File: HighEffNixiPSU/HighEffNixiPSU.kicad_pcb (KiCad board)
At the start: 4 copper layers, 79.9 x 139.9 mm, 74 parts, among them IC1 AZ1117CH-3.3TRG1, J1 Jack-DC, J2 USB_C_Receptacle_USB2.0, Q1 FQD16N25CTM, Q10 2N2219, Q11 2N2219, Q2 2N2219, Q3 2N2219, Q4 2N2219, Q5 2N2219, Q6 2N2219, Q7 2N2219, Q8 2N2219, Q9 2N2219, SW2 EN, U1 LM3478MM, U2 ESP32-S3-MINI-1, U4 HV5622PG, U5 HV5622PG

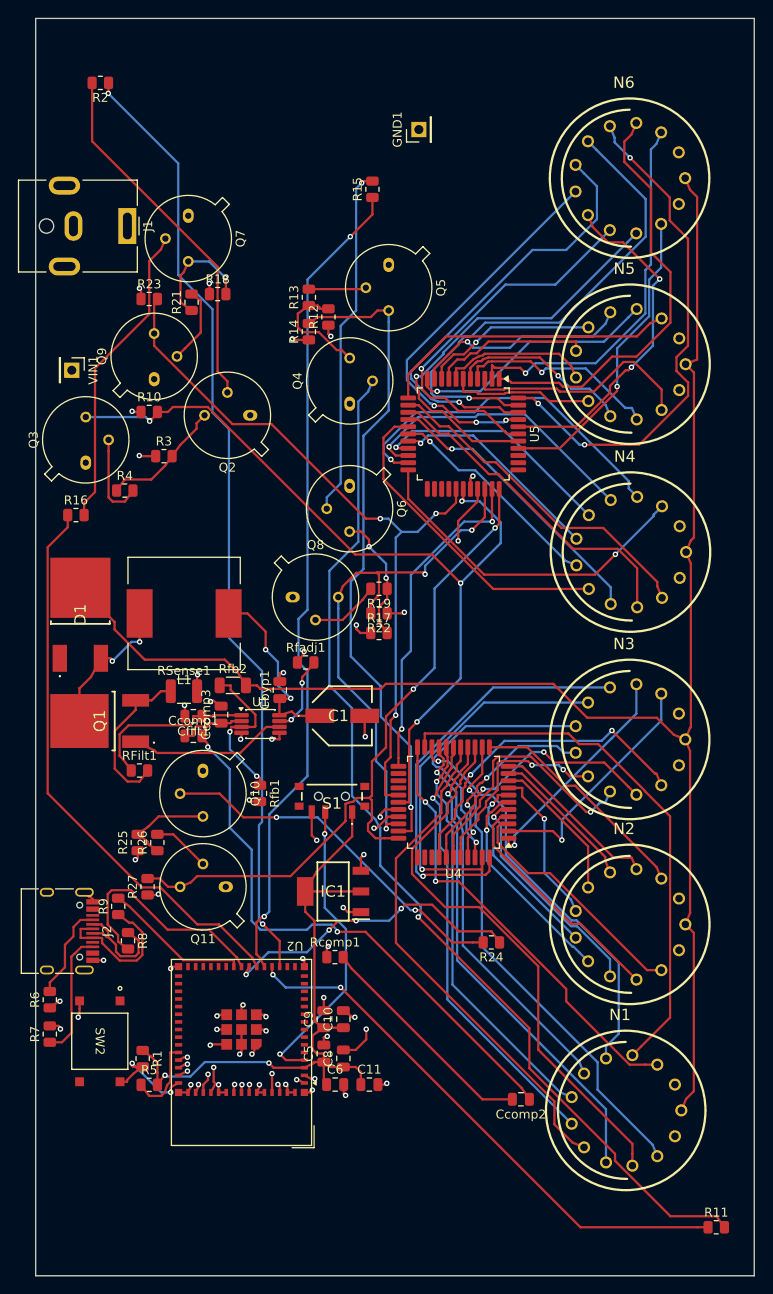
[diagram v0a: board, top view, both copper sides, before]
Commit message: afawj
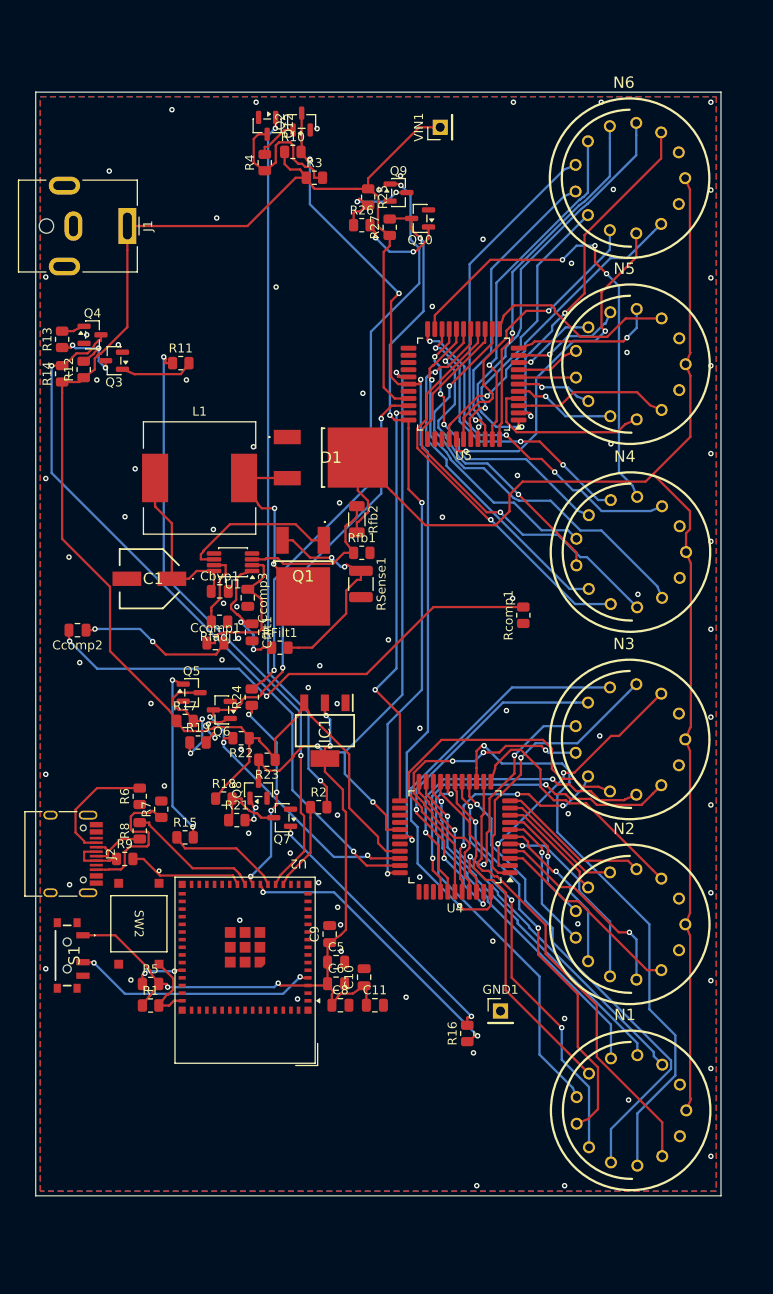
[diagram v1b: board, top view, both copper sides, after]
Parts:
- removed Q11: 2N2219, Package_TO_SOT_THT:TO-39-3
- added Q12: MMBTA06, Package_TO_SOT_SMD:SOT-23, F.Cu at (175.8, 37.0)
- Q10, Q2, Q3, Q4, Q5, Q6, Q7, Q8, Q9: value 2N2219 -> MMBTA06; footprint Package_TO_SOT_THT:TO-39-3 -> Package_TO_SOT_SMD:SOT-23
- moved R11 113.1 mm to (166.1, 63.4)
- moved GND1 98.5 mm to (201.7, 135.5), turned to 0 degrees
- moved R2 84.2 mm to (181.5, 112.8), turned to 0 degrees
- moved R27 78.2 mm to (189.4, 48.3)
- moved R25 76.3 mm to (187.0, 44.9), turned to -90 degrees
- moved R15 75.1 mm to (166.6, 116.2), turned to 0 degrees
- moved R26 72.4 mm to (186.3, 48.1), turned to 0 degrees
- moved R16 72.3 mm to (198.0, 138.0), turned to 90 degrees
- moved Ccomp2 71.8 mm to (154.7, 93.1)
- moved Q7 67.8 mm to (177.4, 114.0), turned to 180 degrees
- moved Q10 66.0 mm to (192.8, 47.3), turned to 180 degrees
- moved R21 57.8 mm to (172.4, 114.3), turned to 0 degrees
- moved R18 56.1 mm to (170.9, 111.9)
- moved R23 52.9 mm to (175.7, 107.5), turned to 180 degrees
- moved Q5 52.4 mm to (167.4, 100.1), turned to 0 degrees
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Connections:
- Q10 pad 1: GND -> Net-(Q10-B)
- Q10 pad 2: Net-(Q10-B) -> GND
- Q10 pad 3: Net-(Q10-C) -> /mcu/BL
- Q2 pad 1: GND -> Net-(Q2-B)
- Q2 pad 2: Net-(Q2-B) -> GND
- Q2 pad 3: Net-(Q2-C) -> /mcu/CLK
- Q3 pad 1: GND -> Net-(Q3-B)
- Q3 pad 2: Net-(Q3-B) -> GND
- Q3 pad 3: /mcu/CLK -> Net-(Q3-C)
- Q4 pad 1: GND -> Net-(Q4-B)
- Q4 pad 2: Net-(Q4-B) -> GND
- Q4 pad 3: Net-(Q4-C) -> /mcu/DAT
- Q5 pad 1: GND -> Net-(Q5-B)
- Q5 pad 2: Net-(Q5-B) -> GND
- Q5 pad 3: /mcu/DAT -> Net-(Q5-C)
- Q6 pad 1: GND -> Net-(Q6-B)
- Q6 pad 2: Net-(Q6-B) -> GND
- Q6 pad 3: Net-(Q6-C) -> /mcu/LE
- Q7 pad 1: GND -> Net-(Q7-B)
- Q7 pad 2: Net-(Q7-B) -> GND
- Q8 pad 1: GND -> Net-(Q8-B)
- Q8 pad 2: Net-(Q8-B) -> GND
- Q8 pad 3: /mcu/LE -> /mcu/POL
- Q9 pad 1: GND -> Net-(Q9-B)
- Q9 pad 2: Net-(Q9-B) -> GND
- Q9 pad 3: /mcu/POL -> Net-(Q9-C)
- R11 pad 2: Net-(Q4-B) -> Net-(Q3-B)
- R12 pad 2: Net-(Q4-C) -> Net-(Q3-C)
- R13 pad 1: Net-(Q4-C) -> Net-(Q3-C)
- R13 pad 2: Net-(Q5-B) -> Net-(Q4-B)
- R15 pad 2: Net-(Q6-B) -> Net-(Q5-B)
- R17 pad 2: Net-(Q6-C) -> Net-(Q5-C)
- R19 pad 1: Net-(Q6-C) -> Net-(Q5-C)
- R19 pad 2: Net-(Q8-B) -> Net-(Q6-B)
- R2 pad 2: Net-(Q2-B) -> Net-(Q12-B)
- R21 pad 2: Net-(Q9-B) -> Net-(Q8-B)
- R24 pad 2: Net-(Q10-B) -> Net-(Q9-B)
- R25 pad 2: Net-(Q10-C) -> Net-(Q9-C)
- R26 pad 1: Net-(Q10-C) -> Net-(Q9-C)
- R26 pad 2: Net-(Q11-B) -> Net-(Q10-B)
- R3 pad 2: Net-(Q2-C) -> Net-(Q12-C)
- R4 pad 1: Net-(Q2-C) -> Net-(Q12-C)
- R4 pad 2: Net-(Q3-B) -> Net-(Q2-B)
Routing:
- net +12V: track 27.1 -> 188.1 mm, vias 13 -> 0
- net Net-(Q4-B): track 117.3 -> 2.57 mm, vias 1 -> 0
- net /mcu/CLK_OUT: track 106.5 -> 9.75 mm, vias 2 -> 0
- net GND: track 81.9 -> 0.00 mm, vias 52 -> 84
- net Net-(Q12-B): track 0.00 -> 79.8 mm, vias 0 -> 2
- net /mcu/LE_OUT: track 92.2 -> 12.6 mm, vias 2 -> 0
- net Net-(Q9-B): track 8.54 -> 66.0 mm, vias 0 -> 2
- net Net-(Ccomp1-Pad2): track 62.7 -> 17.2 mm
- net Net-(Q2-B): track 40.7 -> 4.77 mm
- net Net-(Ccomp2-Pad2): track 25.5 -> 58.4 mm, vias 0 -> 2
- net Net-(Q6-B): track 39.1 -> 6.40 mm, vias 1 -> 2
- net Net-(Q10-B): track 40.6 -> 10.1 mm
- net /mcu/POL_OUT: track 63.3 -> 32.9 mm, vias 0 -> 2
- net VCC: track 182.3 -> 157.2 mm
- net Net-(U4A-HVOUT2): track 61.0 -> 40.2 mm, vias 0 -> 1
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- added copper zone on B.Cu, net GND
- added copper zone on F.Cu, net GND
- removed copper zone on In2.Cu, net +12V
- removed copper zone on In1.Cu, net GND
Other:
- board size 79.9 x 139.9 mm -> 76.2 x 122.8 mm
- copper layers 4 -> 2
